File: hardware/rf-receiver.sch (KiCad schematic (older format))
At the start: 16 parts, among them J1 InputConP6, J3 Raspberry_Pi_2_3, P1 ROT_ENC, U1 TXB0108PWR

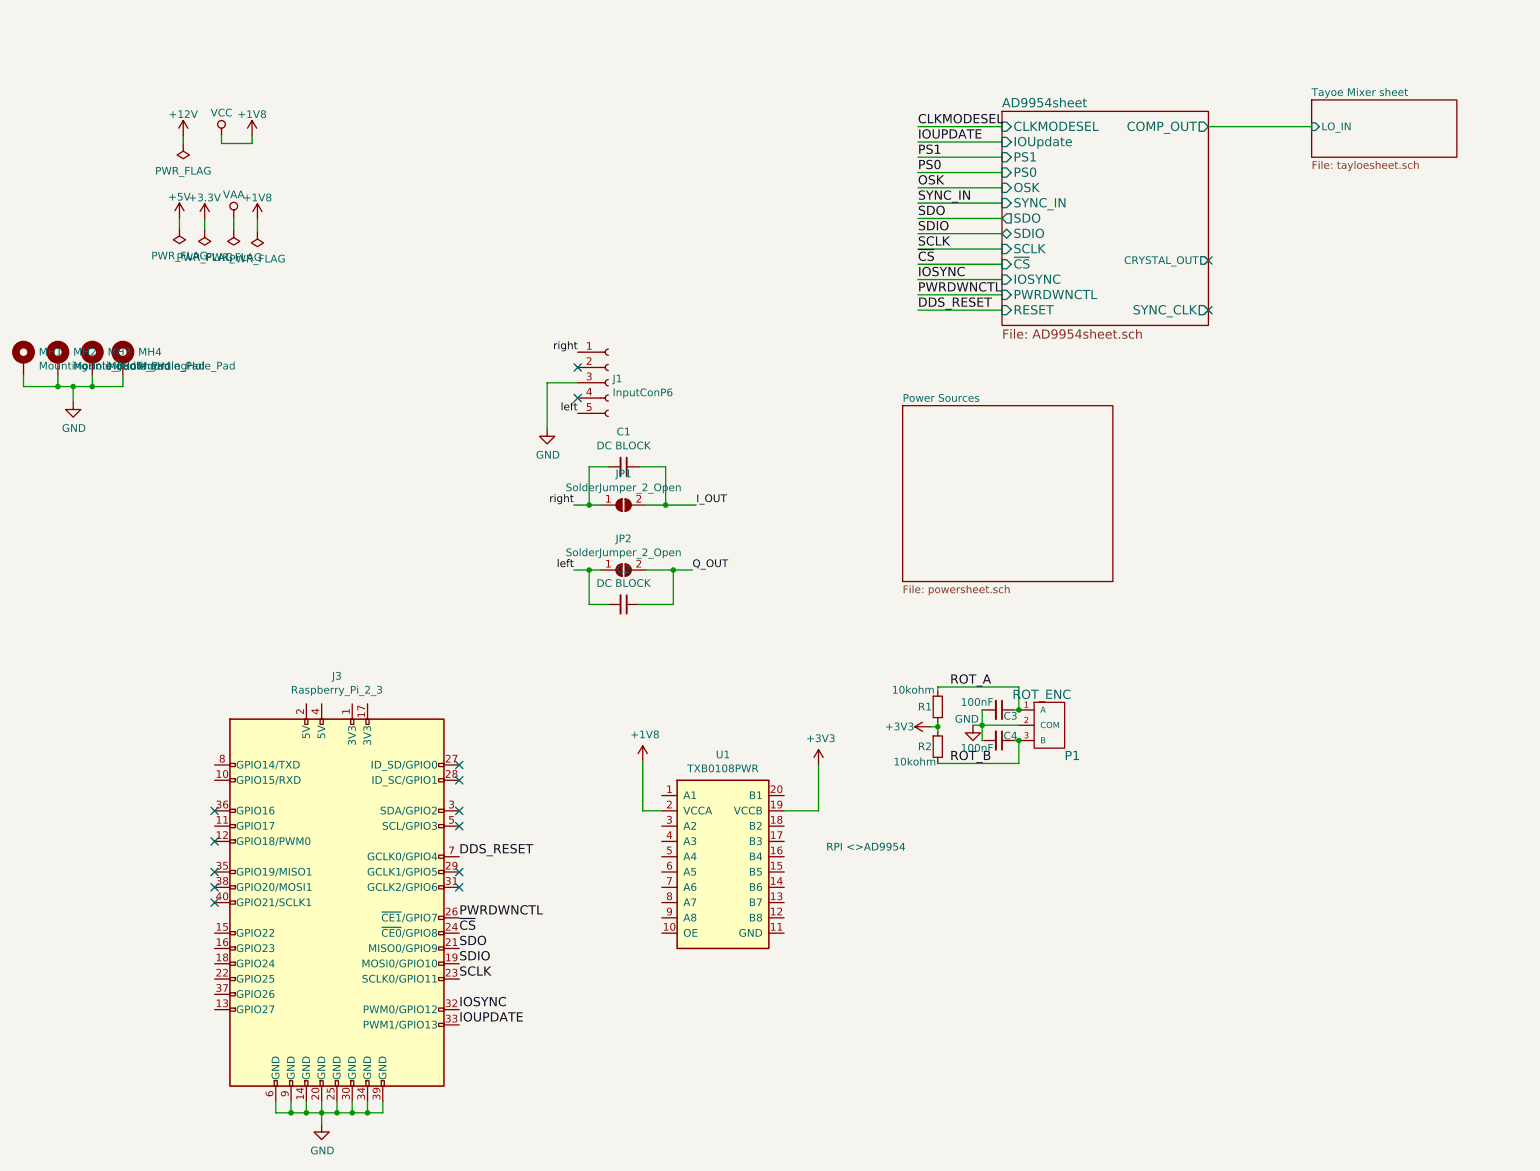
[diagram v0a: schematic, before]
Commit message: Added rpi changes - seems weird that I forgot that for so long
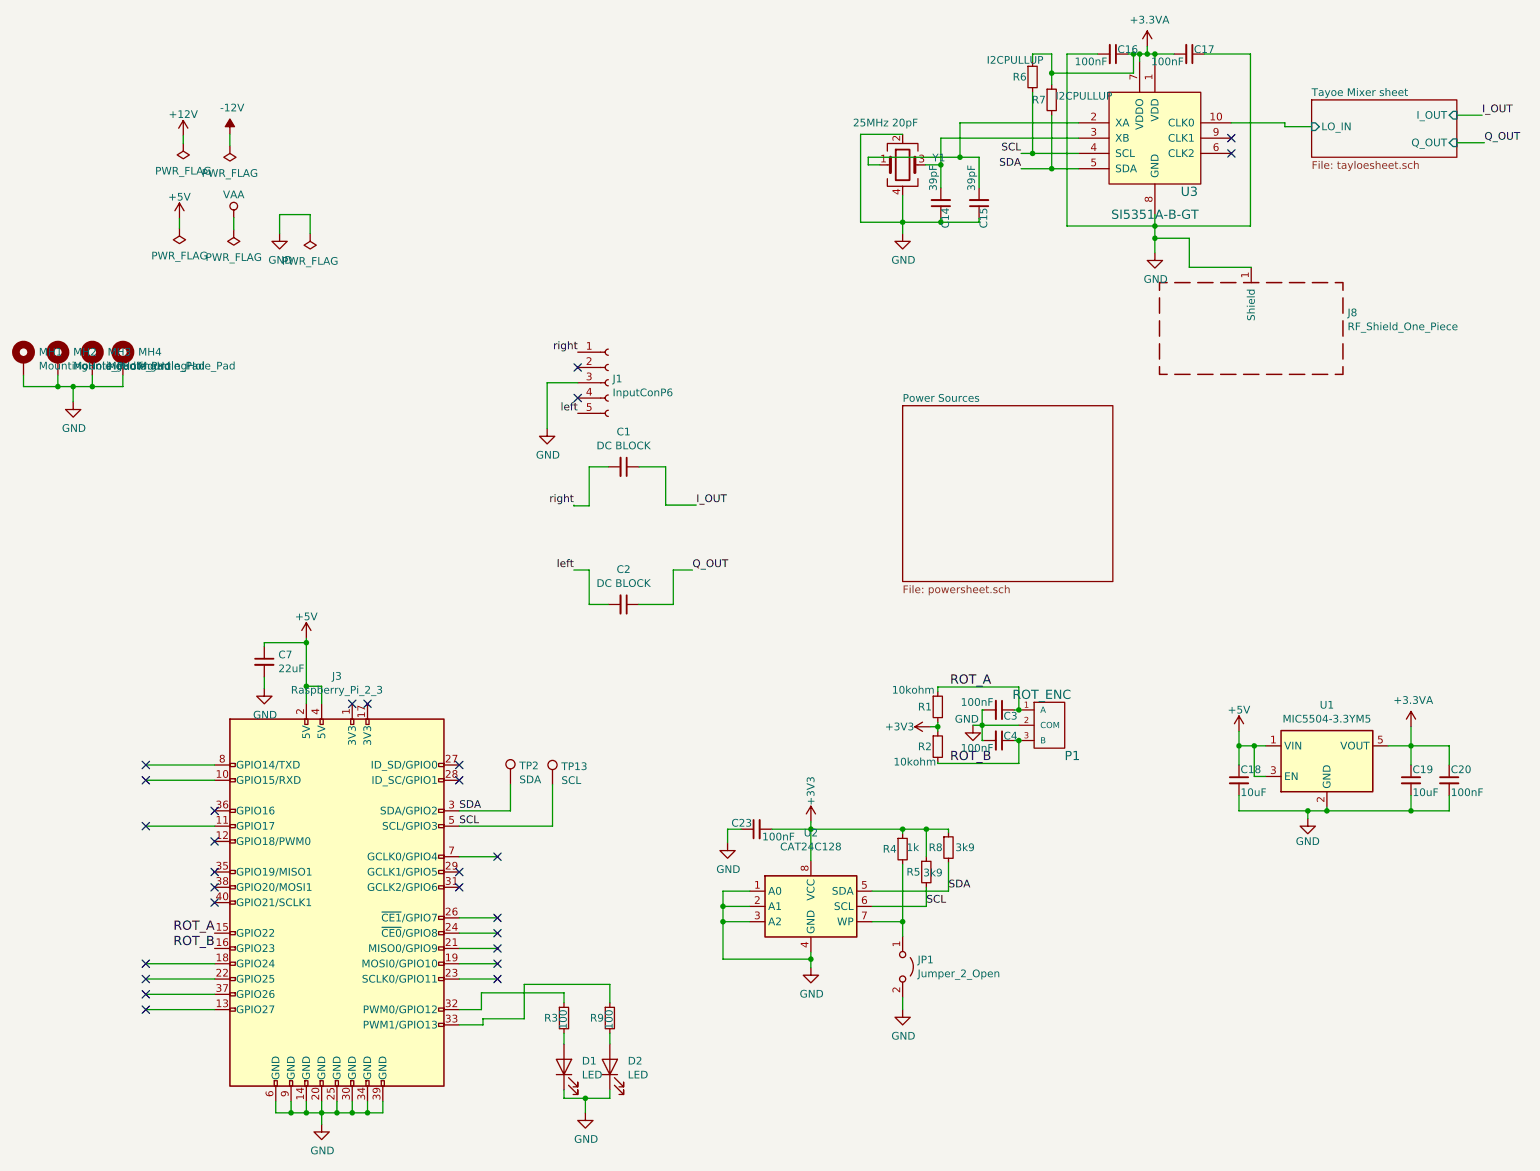
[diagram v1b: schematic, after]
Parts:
- removed JP1, JP2: SolderJumper_2_Open, symbol Jumper:SolderJumper_2_Open
- removed U1: TXB0108PWR, TO_SOT_Packages_SMD:USON-20_2x4mm_Pitch0.4mm, symbol athir:TXB0108PWR
- added C14, C15: 39pF, Capacitor_SMD:C_0603_1608Metric, symbol Device:C_Small
- added C16, C17, C20, C23: 100nF, Capacitor_SMD:C_0603_1608Metric, symbol Device:C_Small
- added C18, C19: 10uF, Capacitor_SMD:C_0603_1608Metric, symbol Device:C_Small
- added C7: 22uF, Capacitor_SMD:C_0805_2012Metric, symbol Device:C_Small
- added D1, D2: LED, Diode_SMD:D_1206_3216Metric, symbol Device:LED
- added J8: RF_Shield_One_Piece, RF_Shielding:Laird_Technologies_BMI-S-101_13.66x12.70mm, symbol Device:RF_Shield_One_Piece
- added JP1: Jumper_2_Open, Connector_PinHeader_2.54mm:PinHeader_1x02_P2.54mm_Vertical, symbol Jumper:Jumper_2_Open
- added R3, R9: 100, Resistor_SMD:R_0805_2012Metric, symbol Device:R_Small
- added R4: 1k, Resistor_SMD:R_0603_1608Metric, symbol Device:R_Small
- added R5, R8: 3k9, Resistor_SMD:R_0603_1608Metric, symbol Device:R_Small
- added R6, R7: I2CPULLUP, Resistor_SMD:R_0603_1608Metric, symbol Device:R_Small
- added TP13: SCL, athir:testpoint_probe, symbol Connector:TestPoint
- added TP2: SDA, athir:testpoint_probe, symbol Connector:TestPoint
- added U1: MIC5504-3.3YM5, Package_TO_SOT_SMD:SOT-23-5, symbol Regulator_Linear:MIC5504-3.3YM5
- added U2: CAT24C128, Package_SO:SOIC-8_3.9x4.9mm_P1.27mm, symbol Memory_EEPROM:CAT24C128
- added U3: SI5351A-B-GT, digikey-footprints:MSOP-10_W3mm, symbol dk_Clock-Timing-Clock-Generators-PLLs-Frequency-Synthesizers:SI5351A-B-GT
- added Y1: 25MHz 20pF, Crystal:Crystal_SMD_3225-4Pin_3.2x2.5mm, symbol Device:Crystal_GND24
- J1: footprint Connector_PinHeader_2.54mm:PinHeader_1x05_P2.54mm_Vertical -> Connector_PinSocket_2.54mm:PinSocket_1x05_P2.54mm_Vertical
- J3: footprint Connector_PinHeader_2.54mm:PinHeader_2x20_P2.54mm_Vertical -> Connector_PinSocket_2.54mm:PinSocket_2x20_P2.54mm_Vertical
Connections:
- net +3V3: now also C23.2, R4.1, R5.1, R8.1, U2.8 (VCC)
- net +5V: now also J3.2 (5V), J3.4 (5V), C18.1, C7.1, U1.1 (VIN), U1.3 (EN)
- net GND: now also C14.1, C15.1, C16.2, C17.1, C18.2, C19.2, C20.2, C23.1, C7.2, D1.1 (K), D2.1 (K), J8.1 (Shield), JP1.2 (B), U1.2 (GND), U2.1 (A0), U2.2 (A1), U2.3 (A2), U2.4 (GND), U3.8 (GND), Y1.2, Y1.4
- net ROT_A: now also J3.15 (GPIO22)
- net ROT_B: now also J3.16 (GPIO23)
- net SDA: now reaches J3.3 (SDA/GPIO2)
- net SDA: now also R7.2, R8.2, TP2.1, U2.5 (SDA), U3.5 (SDA)
- net SCL: now reaches J3.5 (SCL/GPIO3)
- net SCL: now also R5.2, R6.2, TP13.1, U2.6 (SCL), U3.4 (SCL)
- net DDS_RESET: no longer names the net of J3.7 (GCLK0/GPIO4)
- net IOSYNC: no longer names the net of J3.32 (PWM0/GPIO12)
- net IOSYNC: now also R3.1
- net IOUPDATE: no longer names the net of J3.33 (PWM1/GPIO13)
- net IOUPDATE: now also R9.1
- net PWRDWNCTL: no longer names the net of J3.26 (~CE1~/GPIO7)
- net SCLK: no longer names the net of J3.23 (SCLK0/GPIO11)
- net SDIO: no longer names the net of J3.19 (MOSI0/GPIO10)
- net SDO: no longer names the net of J3.21 (MISO0/GPIO9)
- net ~CS: no longer names the net of J3.24 (~CE0~/GPIO8)
- new net: C15.2, U3.2 (XA), Y1.1
- new net: C14.2, U3.3 (XB), Y1.3
- new net: D1.2 (A), R3.2
- new net: JP1.1 (A), R4.2, U2.7 (WP)
- new net: D2.2 (A), R9.2
- new net +3.3VA: C16.1, C17.2, C19.1, C20.1, R6.1, R7.1, U1.5 (VOUT), U3.1 (VDD), U3.7 (VDDO)
- new net Tayoe Mixer sheet/LO_IN: U3.10 (CLK0)
- no-connect marks 15 -> 28
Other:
- note removed: "RPI <>AD9954"
